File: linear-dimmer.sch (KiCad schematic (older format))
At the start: 20 parts, among them P1 POWER, P2 OUTPUT, Q1 Q_NMOS_GDS, U1 LM78L05ACZ, U2 MCP6072, U3 REF3012

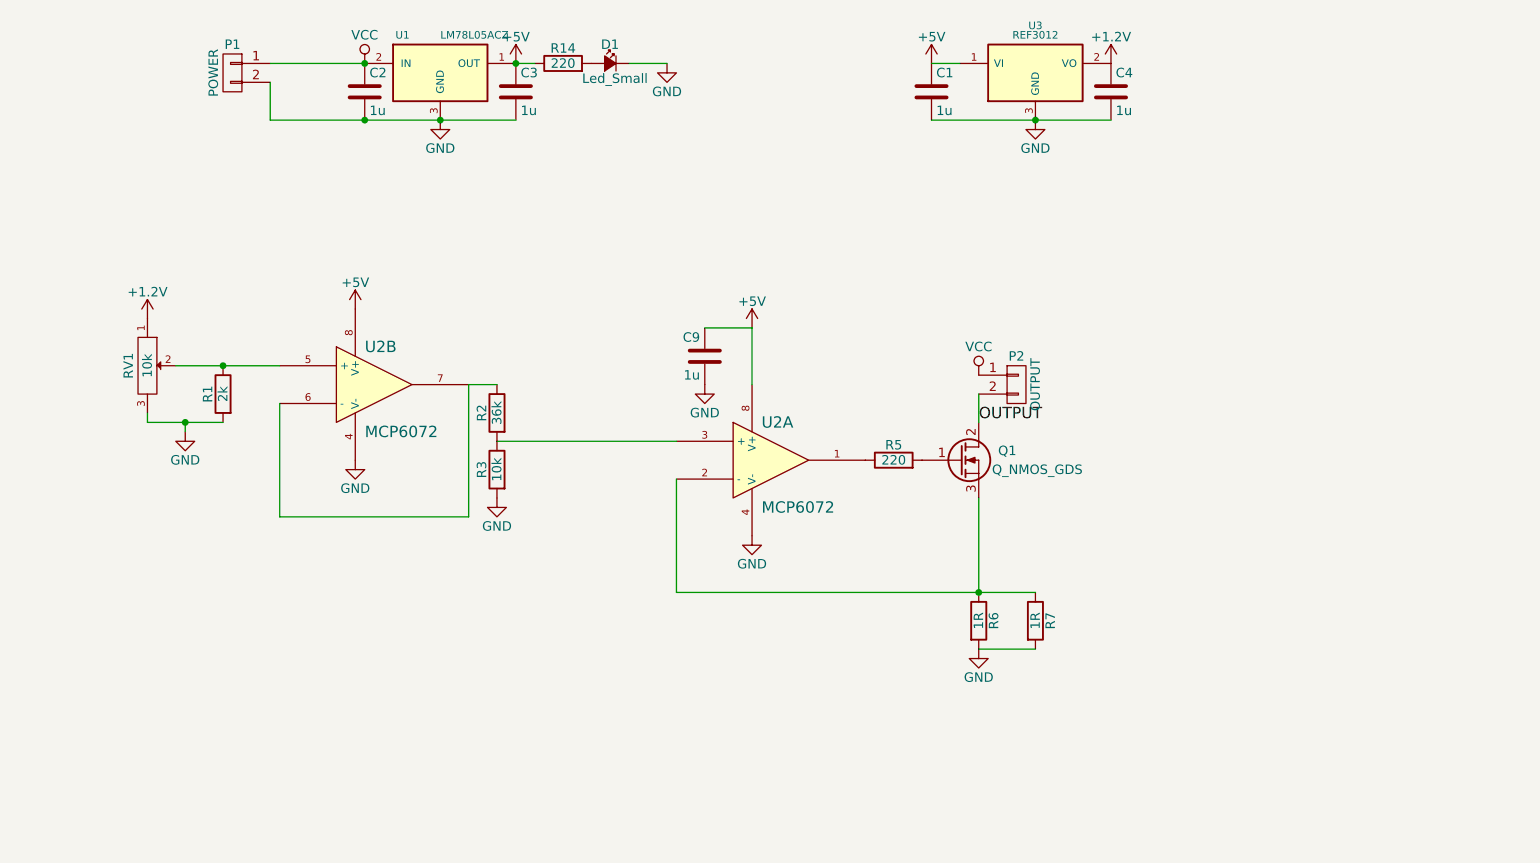
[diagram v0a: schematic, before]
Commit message: Ready to send to PCB house
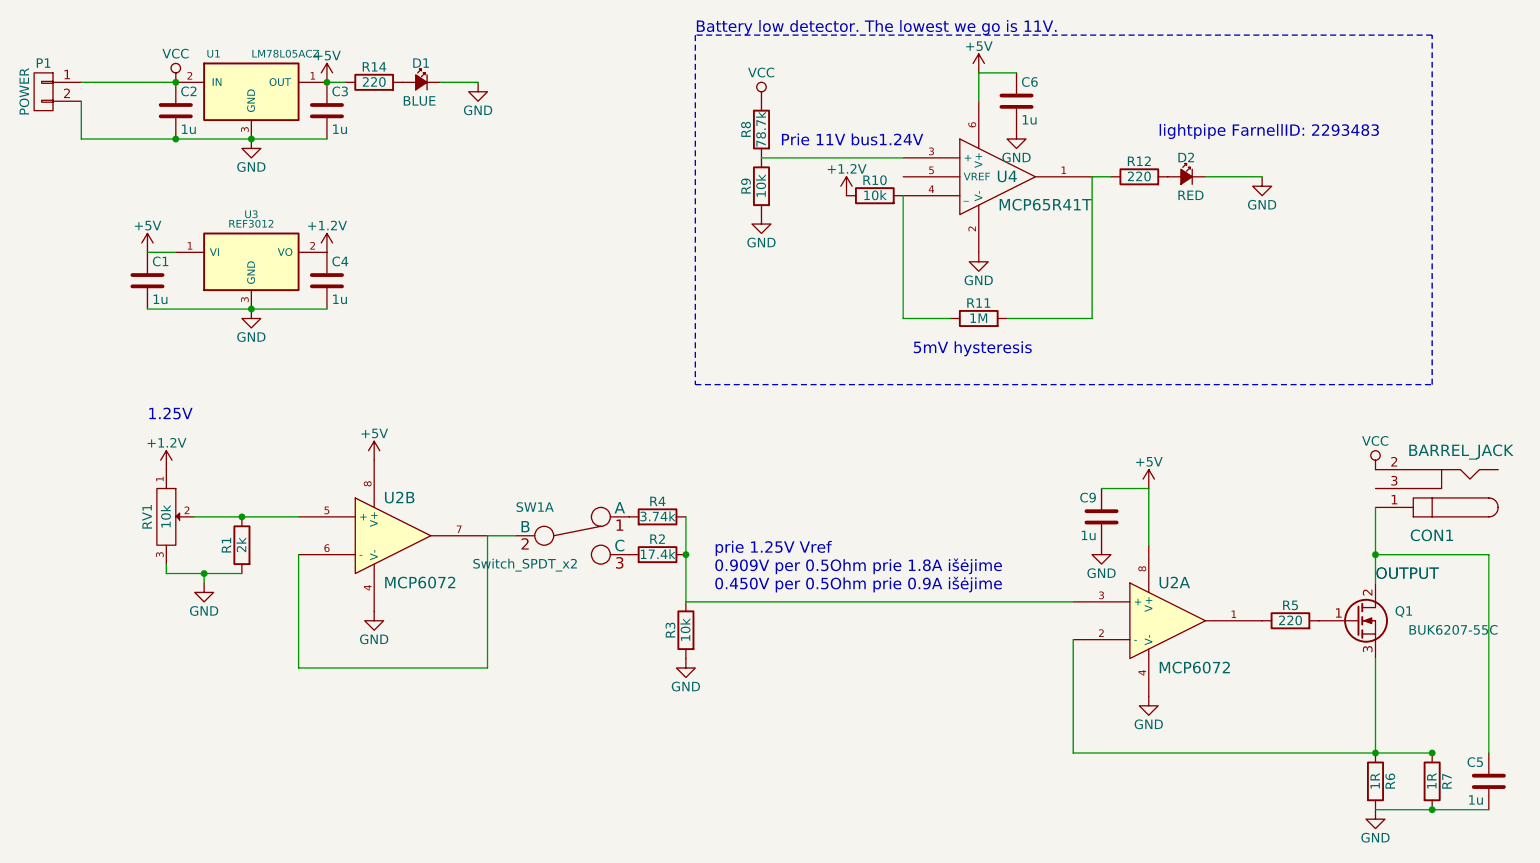
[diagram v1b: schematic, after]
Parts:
- removed P2: OUTPUT, w_pin_strip:pin_socket_2, symbol CONN_01X02
- added C5, C6: 1u, Capacitors_SMD:C_0603_HandSoldering, symbol C
- added CON1: BARREL_JACK, symbol BARREL_JACK
- added D2: RED, w_smd_leds:Led_0603, symbol Led_Small
- added R10, R9: 10k, Resistors_SMD:R_0603_HandSoldering, symbol R
- added R11: 1M, Resistors_SMD:R_0603_HandSoldering, symbol R
- added R12: 220, Resistors_SMD:R_0603_HandSoldering, symbol R
- added R4: 3.74k, Resistors_SMD:R_0603_HandSoldering, symbol R
- added R8: 78.7k, Resistors_SMD:R_0603_HandSoldering, symbol R
- added SW1: Switch_SPDT_x2, Buttons_Switches_SMD:SW_SPDT_PCM12, symbol Switch_SPDT_x2
- added U4: MCP65R41T, w_smd_trans:sot23-6, symbol MCP65R41T-2402
- D1: value Led_Small -> BLUE
- Q1: value Q_NMOS_GDS -> BUK6207-55C; footprint w_smd_trans:sot223 -> w_smd_trans:d-pak; FarnellID 1769679 -> 1863263
- R2: value 36k -> 17.4k
- R6, R7: footprint Resistors_SMD:R_1206_HandSoldering -> Resistors_SMD:R_2512_HandSoldering; FarnellID 1576602 -> 1100070
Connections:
- net +1.2V: now also R10.1
- net +5V: now also C6.1, U4.6 (V+)
- net GND: now also C5.2, C6.2, D2.2 (C), R9.2, U4.2 (V-)
- net OUTPUT: now also C5.1, CON1.1
- net VCC: now also CON1.2, R8.1
- net at U2.6 (-), U2.7: now also SW1.2 (B); no longer R2.1
- net at R3.1, U2.3 (+): now also R2.1, R4.1; no longer R2.2
- new net: R2.2, SW1.3 (C)
- new net: R4.2, SW1.1 (A)
- new net: R11.2, R12.1, U4.1
- new net: D2.1 (A), R12.2
- new net: R8.2, R9.1, U4.3 (+)
- new net: R10.2, R11.1, U4.4 (_)
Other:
- note added: "1.25V"
- note added: "5mV hysteresis"
- note added: "Battery low detector. The lowest we go is 11V."
- note added: "Prie 11V bus1.24V"
- note added: "lightpipe FarnellID: 2293483"
- note added: "prie 1.25V Vref\n0.909V per 0.5Ohm prie 1.8A išėjime\n0.450V per 0.5Ohm prie 0.9A išėjime"
- moved on the sheet: C1, C2, C3, C4, C9, D1, P1, Q1, R1, R14, R2, R3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
